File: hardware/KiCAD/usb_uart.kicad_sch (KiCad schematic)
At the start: 14 parts, among them Q1 BC846B, U2 CP2102N

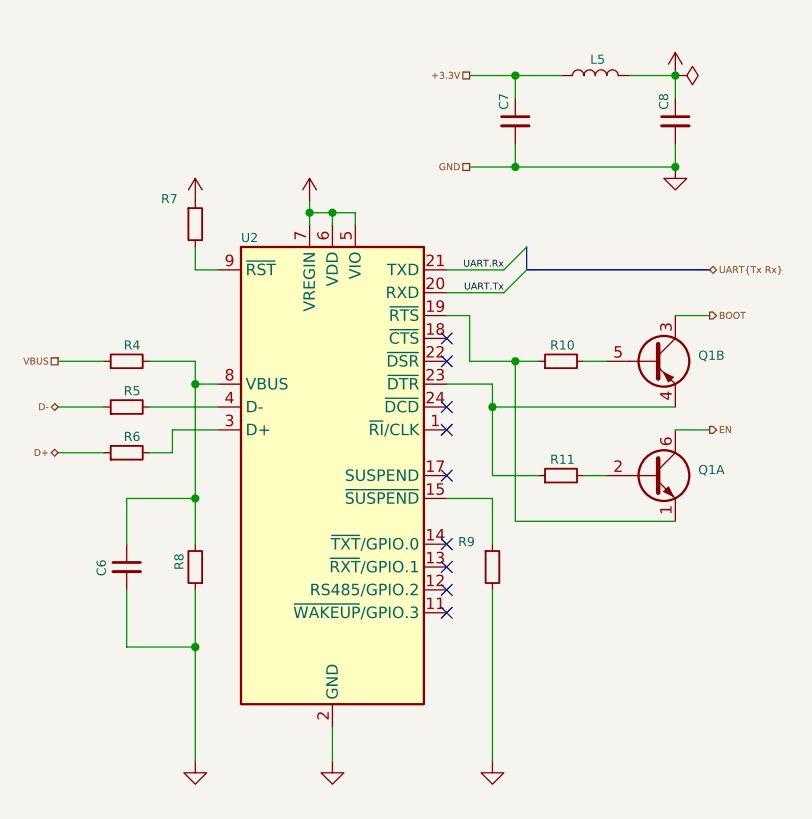
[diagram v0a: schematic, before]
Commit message: update
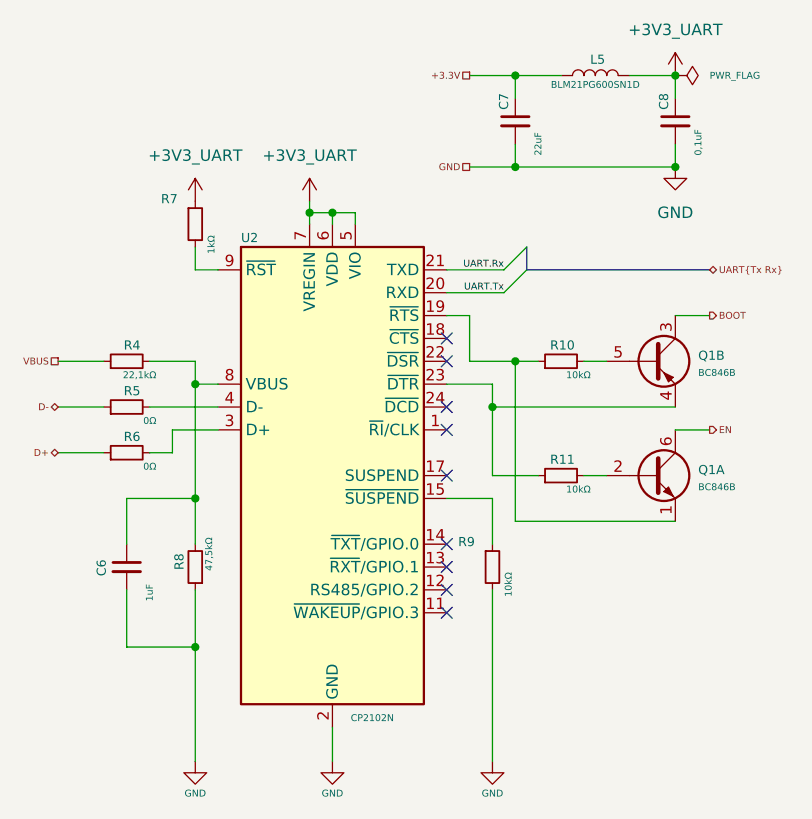
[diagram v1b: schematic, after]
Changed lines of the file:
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@@
 					(size 1.27 1.27)
 				)
-				(hide yes)
 			)
 		)
@@
 				)
 				(justify left)
-				(hide yes)
 			)
 		)
@@
 					(size 1.27 1.27)
 				)
-				(hide yes)
 			)
 		)
@@
 				)
 				(justify left)
-				(hide yes)
 			)
 		)
@@
 					(size 1.27 1.27)
 				)
-				(hide yes)
 			)
 		)
@@
 				)
 				(justify left)
-				(hide yes)
 			)
 		)
@@
 					(size 0.762 0.762)
 				)
-				(hide yes)
 			)
 		)
@@
 				)
 				(justify left)
-				(hide yes)
 			)
 		)
@@
 				)
 				(justify left)
-				(hide yes)
 			)
 		)
@@
 					(size 1.27 1.27)
 				)
-				(hide yes)
 			)
 		)
@@
 				)
 				(justify left)
-				(hide yes)
 			)
 		)
@@
 					(size 0.762 0.762)
 				)
-				(hide yes)
 			)
 		)
@@
 				)
 				(justify left)
-				(hide yes)
 			)
 		)
@@
 				)
 				(justify left)
-				(hide yes)
 			)
 		)
@@
 				)
 				(justify left)
-				(hide yes)
 			)
 		)
@@
 				)
 				(justify left)
-				(hide yes)
 			)
 		)
@@
 					(size 0.762 0.762)
 				)
-				(hide yes)
 			)
 		)
@@
 				)
 				(justify left)
-				(hide yes)
 			)
 		)
@@
 				)
 				(justify left)
-				(hide yes)
 			)
 		)
@@
 				)
 				(justify left)
-				(hide yes)
 			)
 		)
@@
 				)
 				(justify left)
-				(hide yes)
 			)
 		)
@@
 					(size 0.762 0.762)
 				)
-				(hide yes)
 			)
 		)
@@
 				)
 				(justify left)
-				(hide yes)
 			)
 		)
